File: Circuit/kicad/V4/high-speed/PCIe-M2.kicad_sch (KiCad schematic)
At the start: 17 parts, among them J9 Bus_M.2_Socket_M, M1 M.2 Solder Nut, M2 M.2 Solder Nut, M3 M.2 Screw, U6 ASEK-32.768KHZ-L-R-T, U7 AP22815AWU

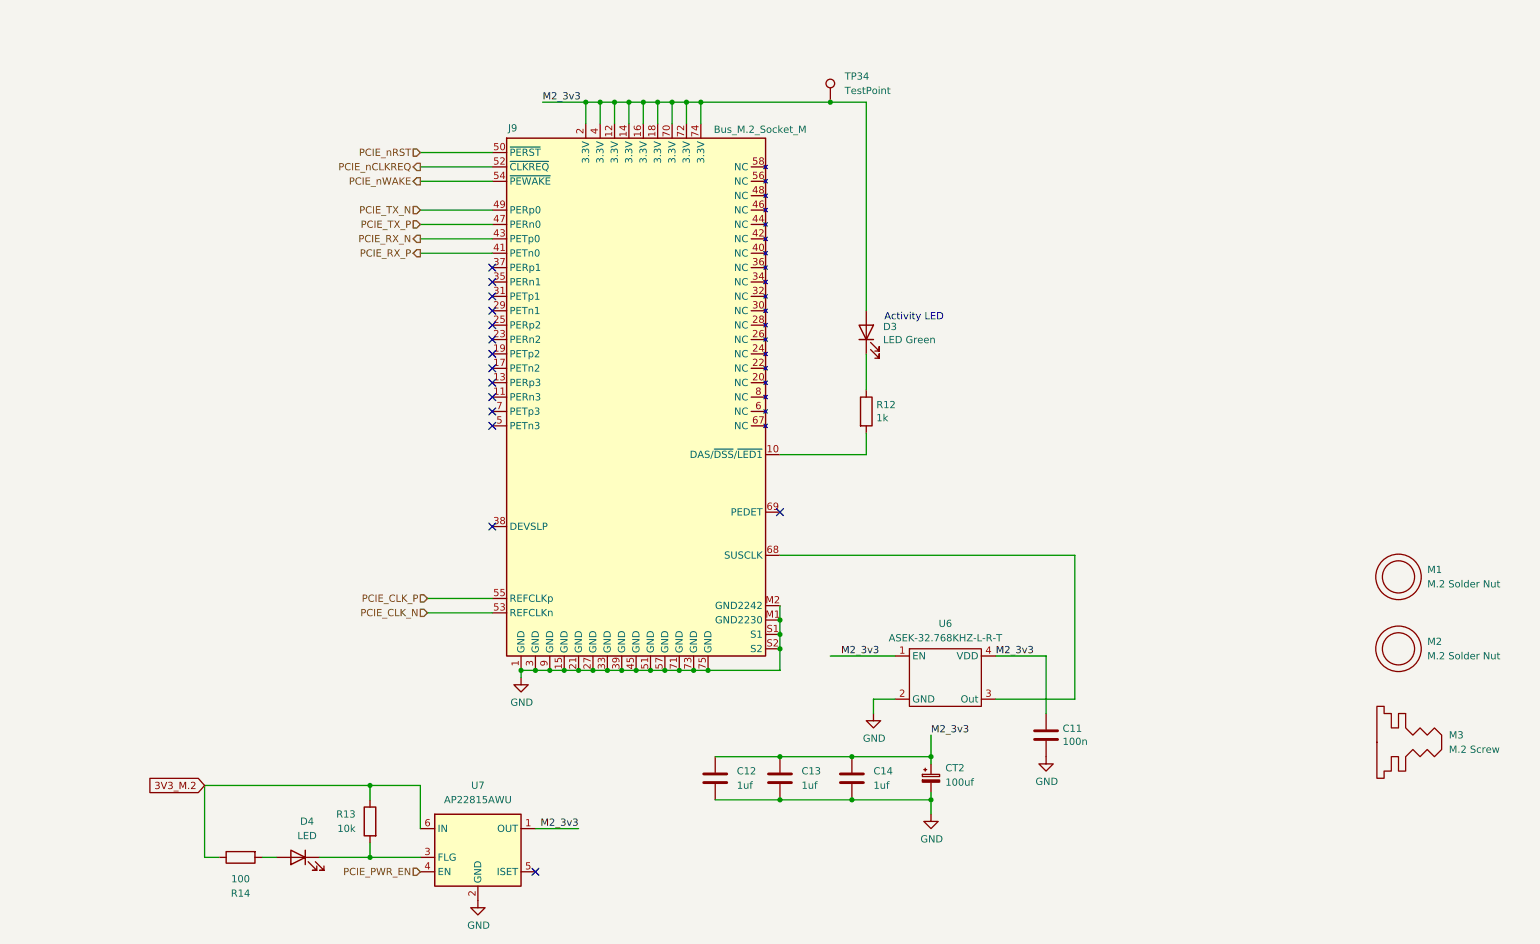
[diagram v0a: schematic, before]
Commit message: kicad: high speed V2.2 Circuit finish psu bom update
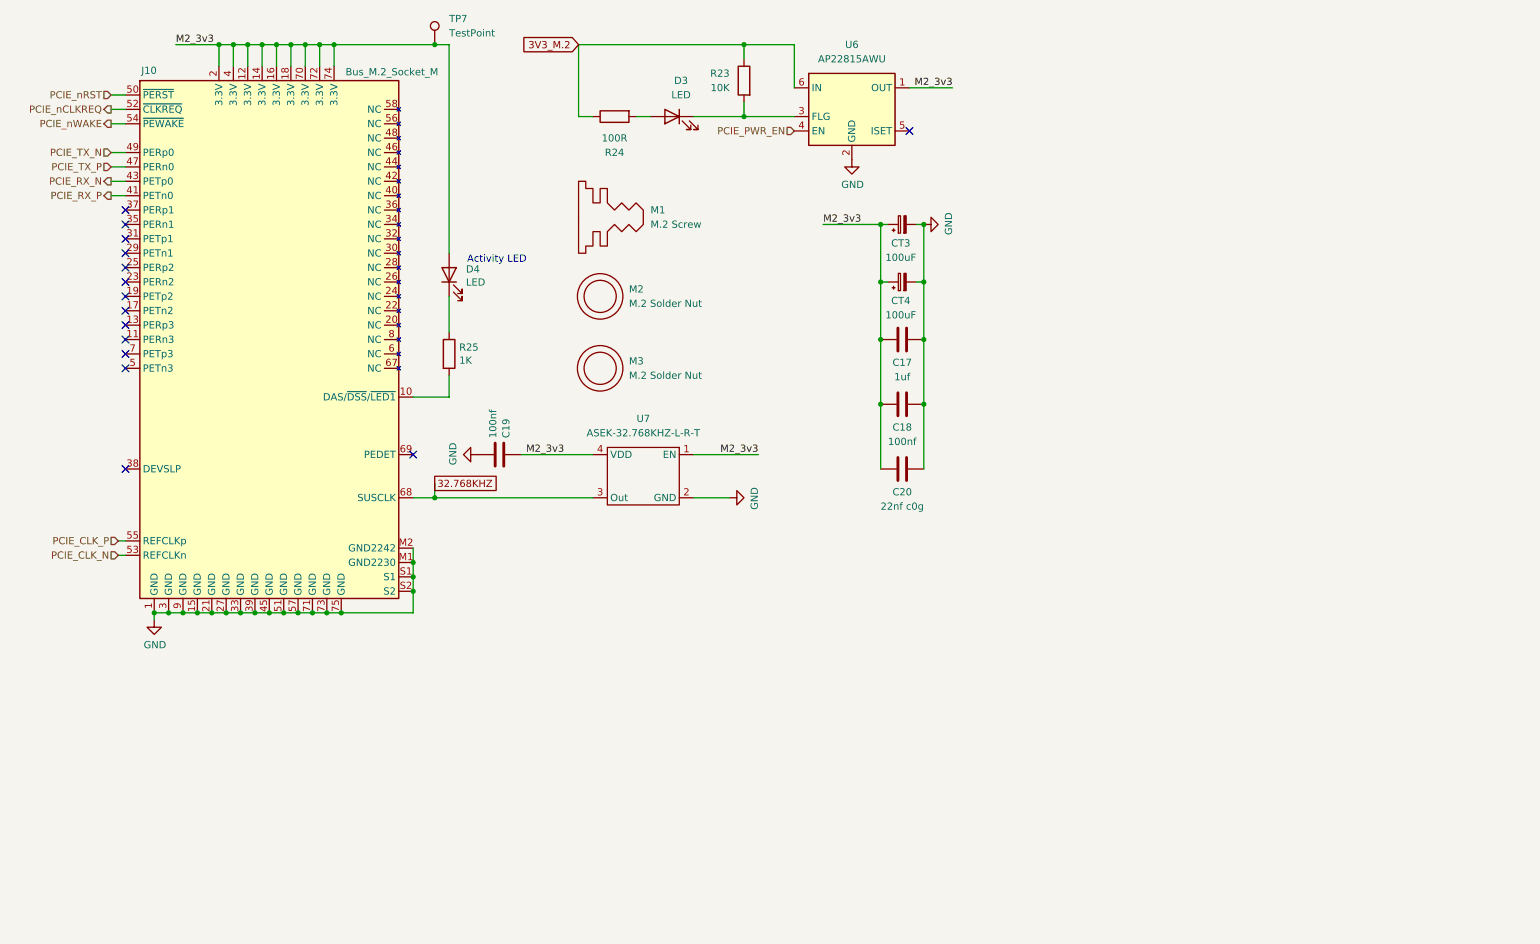
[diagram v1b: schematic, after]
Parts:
- removed C12, C13, C14: 1uf, Capacitor_SMD:C_0805_2012Metric, symbol Device:C
- removed CT2: 100uf, Capacitor_Tantalum_SMD:CP_EIA-7343-31_Kemet-D, symbol Device:C_Polarized_Small
- added C17: 1uf, Capacitor_SMD:C_0805_2012Metric, symbol Device:C
- added C18: 100nf, Capacitor_SMD:C_0805_2012Metric, symbol Device:C
- added C20: 22nf c0g, Capacitor_SMD:C_0805_2012Metric, symbol Device:C
- added CT3, CT4: 100uF, Capacitor_Tantalum_SMD:CP_EIA-7343-31_Kemet-D, symbol Device:C_Polarized_Small
- C19: renamed from C11; value 100n -> 100nf; Cikkszám (none) -> 100.011.22; Field4 Farnell -> (none); Field5 2611911 -> (none); Field6 RM EMK105 B7104KV-F -> (none); Field7 TAIYO YUDEN EUROPE GMBH -> (none); Field8 110091611 -> (none); Link (none) -> https://www.hestore.hu/prod_10001122.html; Part Description 0.1uF 10% 16V Ceramic Capacitor X7R 0402 (1005 Metric) -> (none)
- D3: renamed from D4; Cikkszám (none) -> 100.365.89; Link (none) -> https://www.hestore.hu/prod_10048914.html
- D4: renamed from D3; value LED Green -> LED; Cikkszám (none) -> 100.365.89; Field4 Digikey -> (none); Field5 LTST-S270KGKT -> (none); Field6 SML-A12M8TT86N -> (none); Field7 Rohm -> (none); Field8 650263301 -> (none); Link (none) -> https://www.hestore.hu/prod_10048914.html; Part Description Green 572nm LED Indication - Discrete 2.2V 2-SMD, No Lead -> (none)
- J10: renamed from J9; footprint psu:M.2 M Key socket -> panel:M.2 M Key socket; Cikkszám (none) -> 523-MDT420M03001; Field5 MTSSD03-67MSW337 -> (none); Field6 MTSSD03-67MSW337 -> (none); Field7 MTCONN -> (none); Link (none) -> https://hu.mouser.com/ProductDetail/Amphenol-FCI/MDT420M030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; Part Description M.2 M Key connector -> (none)
- M1: renamed from M3; Cikkszám (none) -> -; Link (none) -> -; Part Description M.2 Screw -> (none); now left out of the parts list
- M2: renamed from M1; Cikkszám (none) -> -; Link (none) -> -; Part Description Solder nut for M.2 slot -> (none); now left out of the parts list
- M3: renamed from M2; Cikkszám (none) -> -; Link (none) -> -; Part Description Solder nut for M.2 slot -> (none); now left out of the parts list
- R23: renamed from R13; value 10k -> 10K; Cikkszám (none) -> 100.011.45; Link (none) -> https://www.hestore.hu/prod_10001145.html
- R24: renamed from R14; value 100 -> 100R; Cikkszám (none) -> 100.011.42; Link (none) -> https://www.hestore.hu/prod_10001142.html
- R25: renamed from R12; value 1k -> 1K; Cikkszám (none) -> 100.011.57; Field4 Farnell -> (none); Field5 9239235 -> (none); Field6 RK73H1ETTP1001F -> (none); Field7 KOA EUROPE GMBH -> (none); Field8 125049511 -> (none); Link (none) -> https://www.hestore.hu/prod_10001157.html; Part Description Resistor 1K M1005 1% 63mW -> (none)
- TP7: renamed from TP34; Cikkszám (none) -> -; Link (none) -> -; now left out of the parts list
- U6: renamed from U7; Cikkszám (none) -> 100.491.23; Link (none) -> https://www.hestore.hu/prod_10049123.html
- U7: renamed from U6; Cikkszám (none) -> 100.491.02; Field5 ASEK-32.768KHZ-L-R-T -> (none); Field6 ASEK-32.768KHZ-L-R-T -> (none); Field7 abracon -> (none); Link (none) -> https://www.hestore.hu/prod_10049102.html; Part Description 32KHz Xtal oscilator -> (none)
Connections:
- net GND: now also C17.2, C18.2, C20.2, CT3.2, CT4.2
- net M2_3v3: now also C17.1, C18.1, C20.1, CT3.1, CT4.1
- net 32.768KHZ: now reaches J10.68 (SUSCLK), U7.3 (Out)
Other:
- moved on the sheet: C19, D3, D4, J10, M1, M2, M3, R23, R24, R25, TP7, U6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
